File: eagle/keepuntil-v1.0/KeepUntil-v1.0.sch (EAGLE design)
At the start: 12 parts, among them Q1 CSTCR6M00G53Z, U1 ATMEGA328P-AU

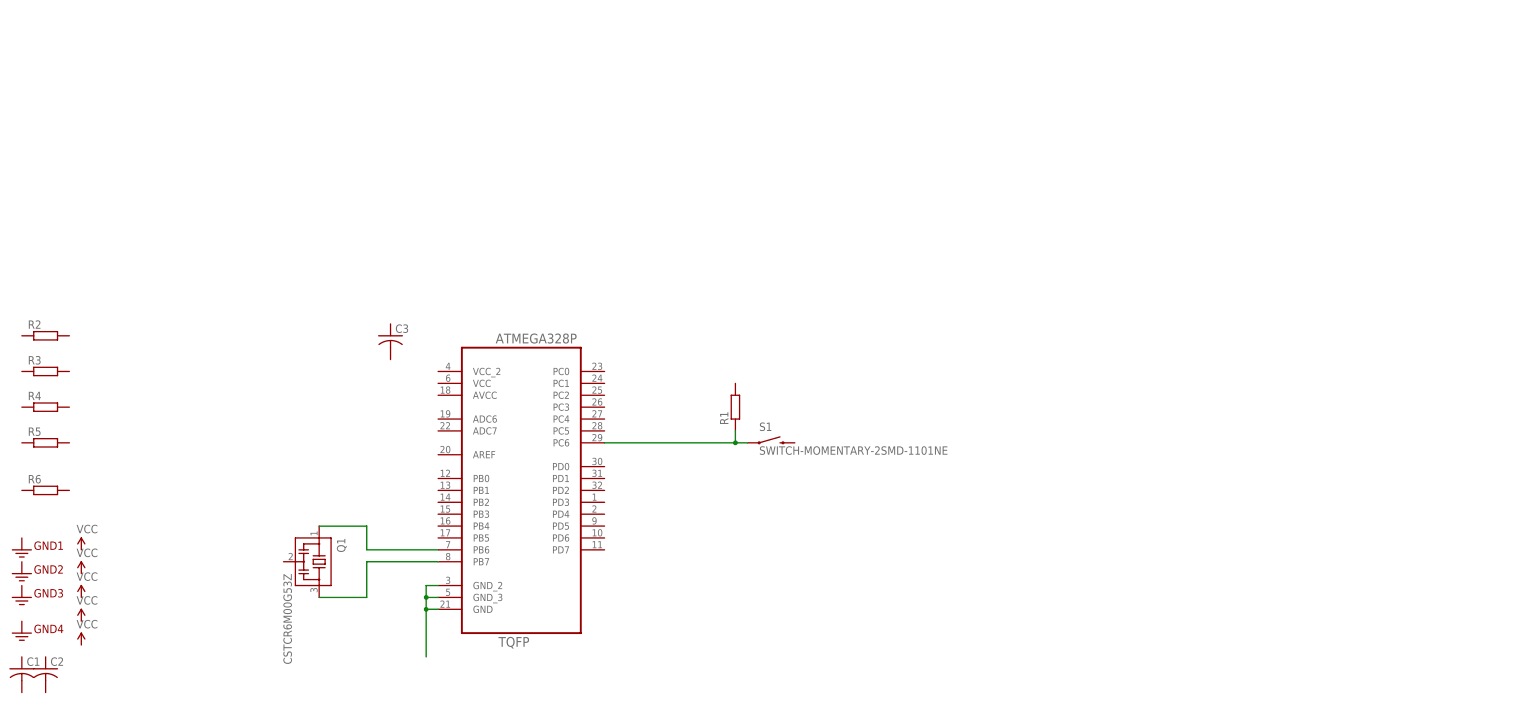
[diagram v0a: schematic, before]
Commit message: schematic work
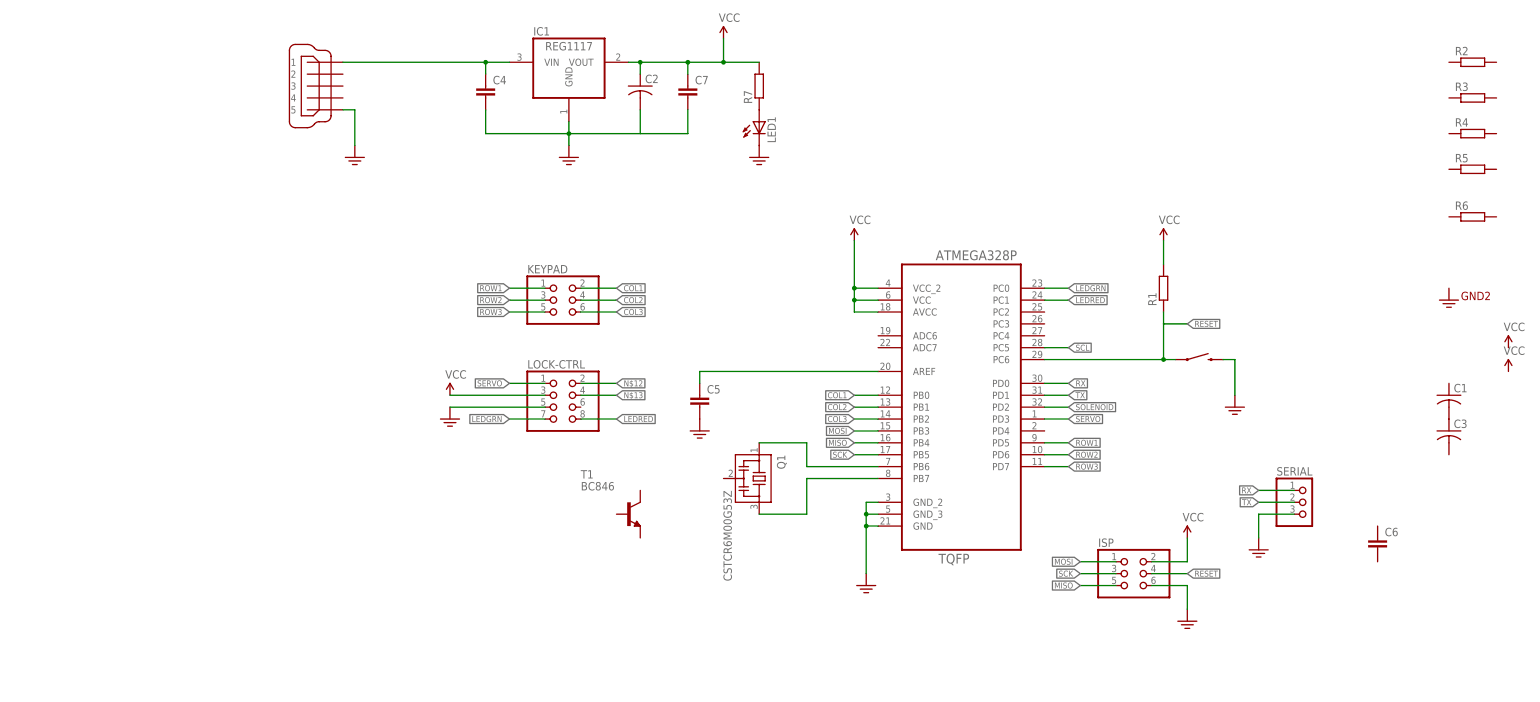
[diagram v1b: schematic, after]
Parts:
- added C4, C5, C6, C7: (no value), resistor:C-EUC0805
- added IC1: REG1117, burr-brown:REG1117
- added ISP, KEYPAD: (no value), pinhead:PINHD-2X3
- added LED1: (no value), led:LEDSMT1206
- added LOCK-CTRL: (no value), pinhead:PINHD-2X4
- added R7: (no value), resistor:R-EU_R0805
- added SERIAL: (no value), pinhead:PINHD-1X3
- added T1: BC846, transistor:BC846
- added X1: MINI-USB-32005-201, con-cypressindustries:MINI-USB-32005-201
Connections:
- removed net N$3: R1.1, S1.1, U1.PC6
- new net 3.3V: C2.2, C4.2, C5.2, C7.2, IC1.GND, ISP.6, LED1.C, S1.2, SERIAL.3, X1.5
- new net COL1: KEYPAD.2, U1.PB0
- new net COL2: KEYPAD.4, U1.PB1
- new net COL3: KEYPAD.6, U1.PB2
- new net LEDGRN: LOCK-CTRL.7, U1.PC0
- new net LEDRED: LOCK-CTRL.8, U1.PC1
- new net MISO: ISP.5, U1.PB4
- new net MOSI: ISP.1, U1.PB3
- new net N$12: LOCK-CTRL.2
- new net N$13: LOCK-CTRL.4
- new net N$5: C4.1, IC1.VIN, X1.1
- new net N$6: C1.2, C3.1
- new net N$7: LED1.A, R7.1
- new net N$8: C5.1, U1.AREF
- new net N$9: LOCK-CTRL.5
- new net RESET: ISP.4, R1.1, S1.1, U1.PC6
- new net ROW1: KEYPAD.1, U1.PD5
- new net ROW2: KEYPAD.3, U1.PD6
- new net ROW3: KEYPAD.5, U1.PD7
- new net RX: SERIAL.1, U1.PD0
- new net SCK: ISP.3, U1.PB5
- new net SCL: U1.PC5
- new net SERVO: LOCK-CTRL.1, U1.PD3
- new net SOLENOID: U1.PD2
- new net TX: SERIAL.2, U1.PD1
- new net VCC: C2.1, C7.1, IC1.VOUT, ISP.2, LOCK-CTRL.3, R1.2, R7.2, U1.AVCC, U1.VCC, U1.VCC_2
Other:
- moved on the sheet: C1, C2, C3, Q1, R1, R2, R3, R4, R5, R6
